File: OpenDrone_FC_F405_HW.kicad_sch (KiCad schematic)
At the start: 88 parts, among them J1 Conn_01x05, J11 Conn_01x05, J12 Conn_01x05, J13 Conn_01x02, J14 Conn_01x02, J16 Conn_01x05, J17 Conn_02x03_Odd_Even, J2 Conn_01x02, J3 Conn_01x02, J4 Conn_01x02, J5 Conn_01x02, J6 Conn_01x08, J7 Conn_01x02, J8 Conn_01x04, J9 Conn_01x02, U1 STM32F405RGTx, U2 TPS54331, U4 MPU6000, U5 HMC5883L, U6 BMP280, U7 TPS54331, U8 Board, Y2 8Mhz

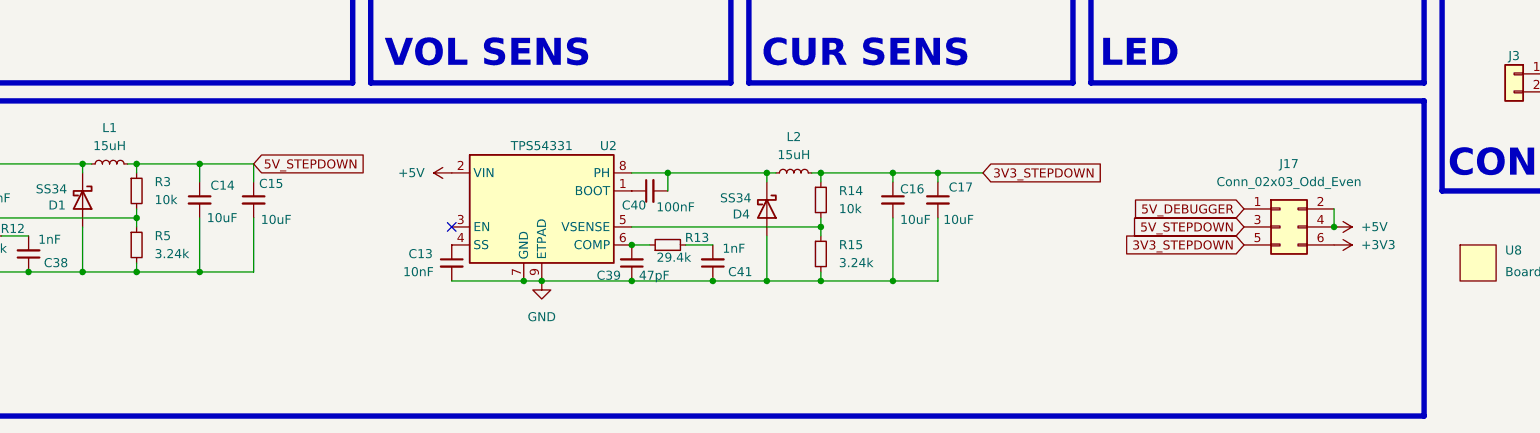
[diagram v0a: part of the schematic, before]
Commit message: update project
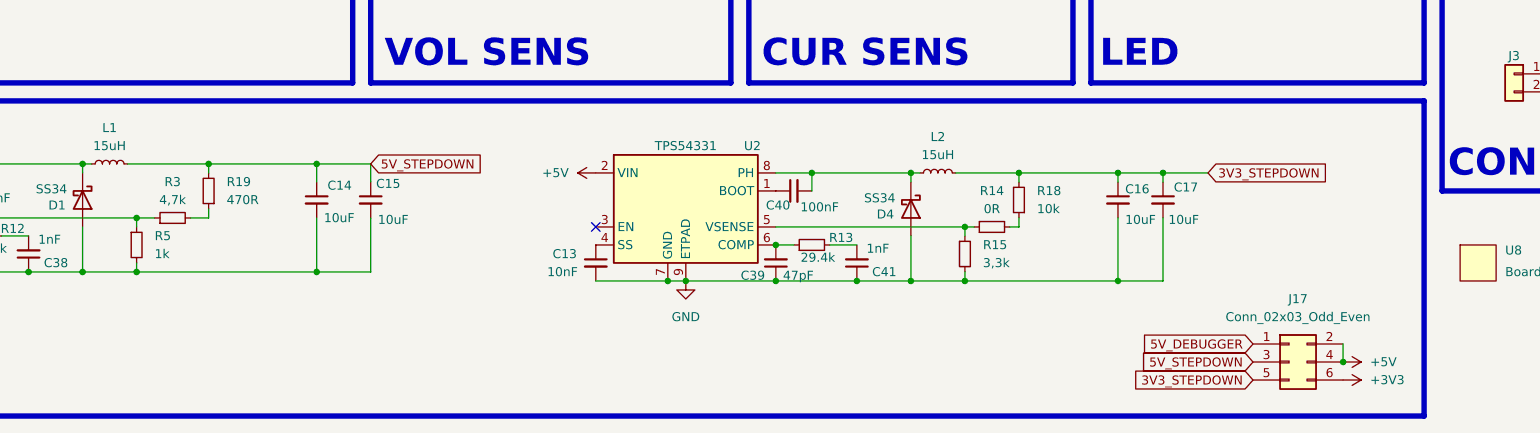
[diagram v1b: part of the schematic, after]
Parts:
- added R18: 10k, Resistor_SMD:R_0402_1005Metric, symbol Device:R_Small
- added R19: 470R, Resistor_SMD:R_0402_1005Metric, symbol Device:R_Small
- R14: value 10k -> 0R
- R15: value 3.24k -> 3,3k
- R3: value 10k -> 4,7k
- R5: value 3.24k -> 1k
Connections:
- net 3V3_STEPDOWN: now also R18.2; no longer R14.1
- net 5V_STEPDOWN: now also R19.2; no longer R3.1
- net at R15.1, U2.5 (VSENSE): now also R14.1; no longer R14.2
- net at R5.1, U7.5 (VSENSE): now also R3.1; no longer R3.2
- new net: R14.2, R18.1
- new net: R19.1, R3.2
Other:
- moved on the sheet: C13, C14, C15, C16, C17, C39, C40, C41, D4, J17, L2, R13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

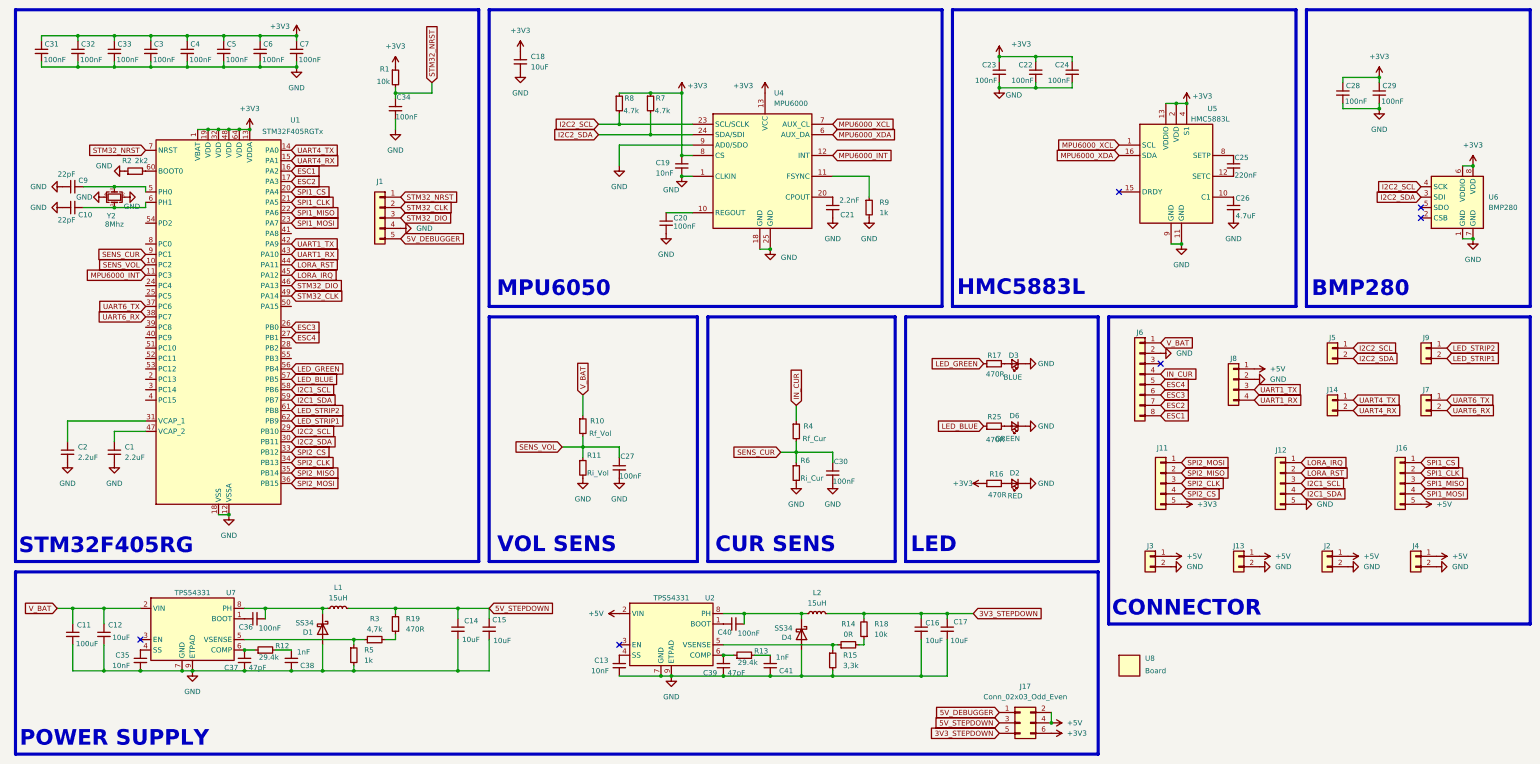
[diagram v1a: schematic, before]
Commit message: update project
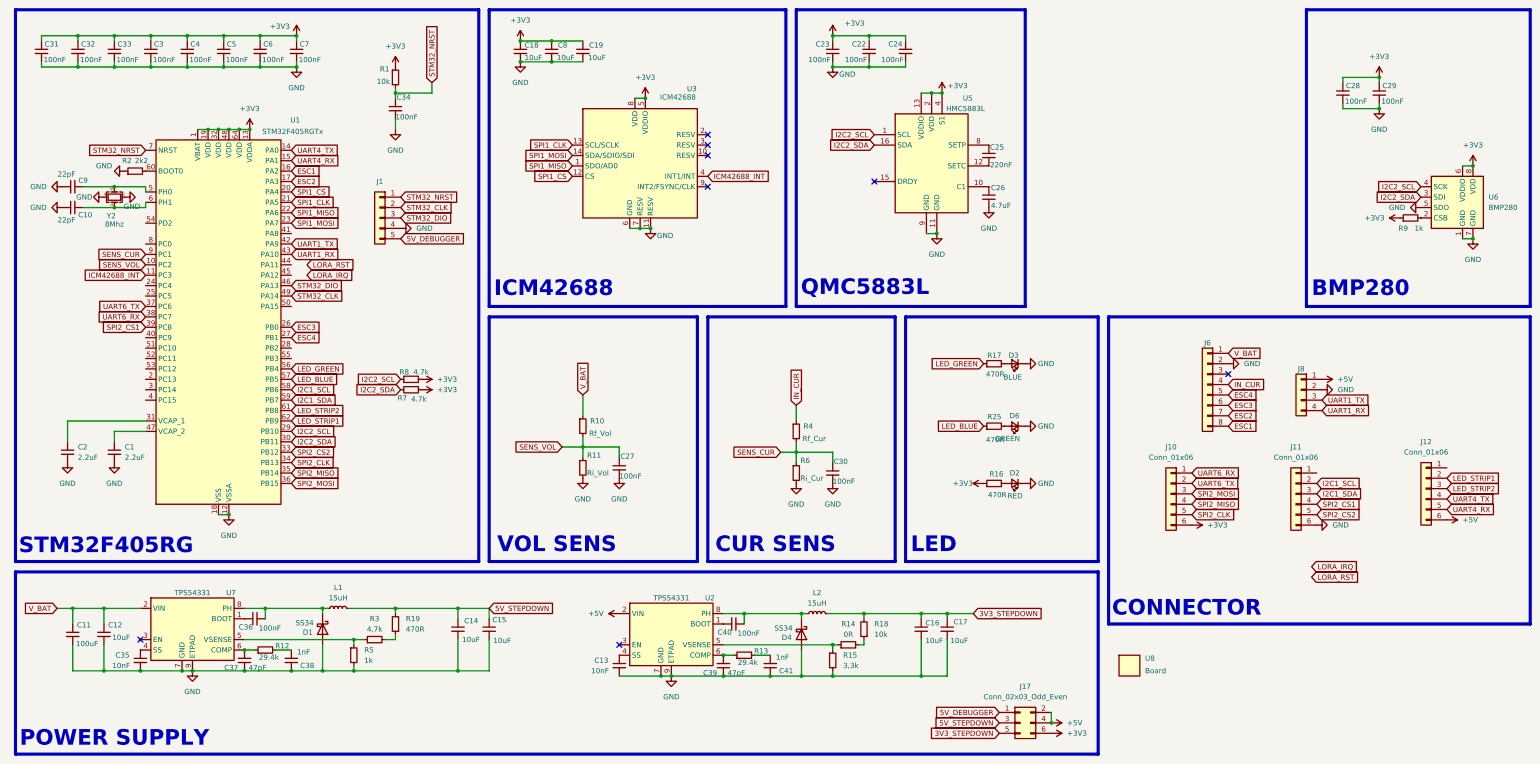
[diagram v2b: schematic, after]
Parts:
- removed C20: 100nF, Capacitor_SMD:C_0402_1005Metric, symbol Device:C_Small
- removed C21: 2.2nF, Capacitor_SMD:C_0402_1005Metric, symbol Device:C_Small
- removed J11, J12, J16: Conn_01x05, Footprint:Header_1x05_P2.00mm_Vertical, symbol Connector_Generic:Conn_01x05
- removed J13, J14, J2, J3, J4, J5, J7, J9: Conn_01x02, Footprint:HolePad_1x2, symbol Connector_Generic:Conn_01x02
- removed U4: MPU6000, Footprint:QFN-24-1EP_4x4mm_P0.5mm_EP2.15x2.15mm, symbol MPU6000:MPU6000
- added C8: 10uF, Capacitor_SMD:C_0402_1005Metric, symbol Device:C_Small
- added J10, J11, J12: Conn_01x06, Footprint:Header_1x06_P2.00mm_Vertical, symbol Connector_Generic:Conn_01x06
- added U3: ICM42688, Package_LGA:LGA-14_3x2.5mm_P0.5mm_LayoutBorder3x4y, symbol ICM42688:ICM42688
- C19: value 10nF -> 10uF
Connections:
- net MPU6000_XCL is gone; now on net I2C2_SCL: U5.1 (SCL)
- net MPU6000_XDA is gone; now on net I2C2_SDA: U5.16 (SDA)
- net +3V3: now also R8.2, R9.1, C8.1, J10.6 (Pin_6), U3.5 (VDDIO), U3.8 (VDD); no longer R8.1
- net +5V: now also J12.6 (Pin_6)
- net GND: now also U6.5 (SDO), C8.2, J11.6 (Pin_6), U3.11 (RESV), U3.6 (GND), U3.7 (RESV); no longer R9.2
- net I2C1_SCL: now also J11.2 (Pin_2)
- net I2C1_SDA: now also J11.3 (Pin_3)
- net I2C2_SCL: now also R8.1; no longer R8.2
- net LED_STRIP1: now also J12.2 (Pin_2)
- net LED_STRIP2: now also J12.3 (Pin_3)
- net LORA_IRQ: no longer U1.45 (PA12)
- net LORA_RST: no longer U1.44 (PA11)
- net SPI1_CLK: now also U3.13 (SCL/SCLK)
- net SPI1_CS: now also U3.12 (CS)
- net SPI1_MISO: now also U3.1 (SDO/AD0)
- net SPI1_MOSI: now also U3.14 (SDA/SDIO/SDI)
- net SPI2_CLK: now also J10.5 (Pin_5)
- net SPI2_MISO: now also J10.4 (Pin_4)
- net SPI2_MOSI: now also J10.3 (Pin_3)
- net UART4_RX: now also J12.5 (Pin_5)
- net UART4_TX: now also J12.4 (Pin_4)
- net UART6_RX: now also J10.1 (Pin_1)
- net UART6_TX: now also J10.2 (Pin_2)
- net at U6.2 (CSB): now also R9.2
- net SPI2_CS1: now reaches U1.39 (PC8)
- net SPI2_CS1: now also J11.4 (Pin_4)
- net MPU6000_INT renamed ICM42688_INT
- net ICM42688_INT: now also U3.4 (INT1/INT)
- net SPI2_CS renamed SPI2_CS2
- net SPI2_CS2: now also J11.5 (Pin_5)
- no-connect marks 6 -> 8
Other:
- note added: "ICM42688"
- note added: "QMC5883L"
- note removed: "HMC5883L"
- note removed: "MPU6050"
- moved on the sheet: C18, C22, C23, C24, C25, C26, J6, J8, R7, R8, R9, U5

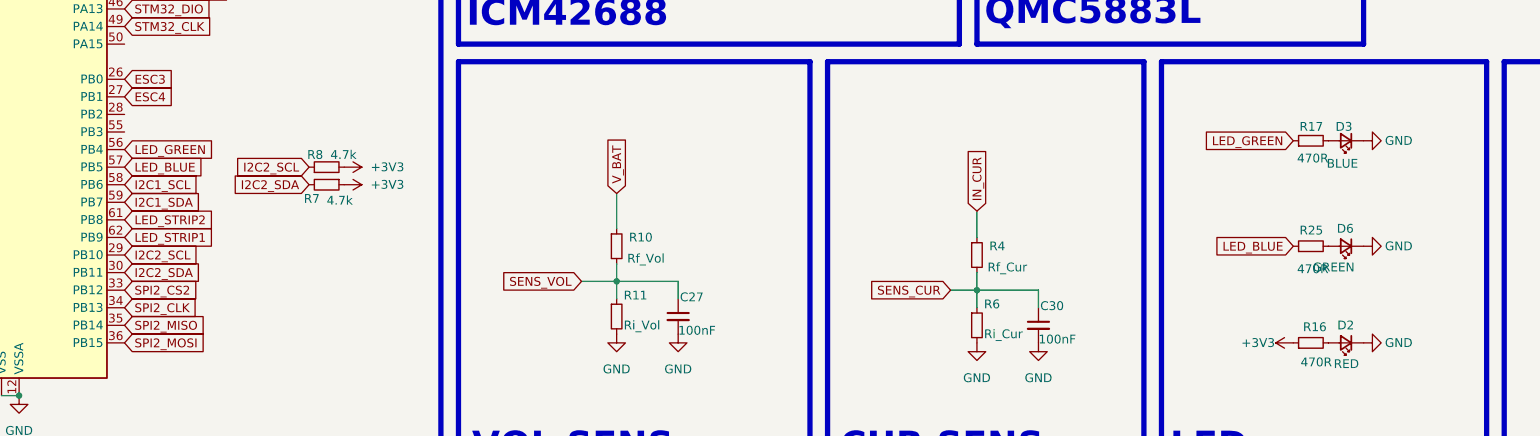
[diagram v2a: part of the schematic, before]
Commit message: update routing
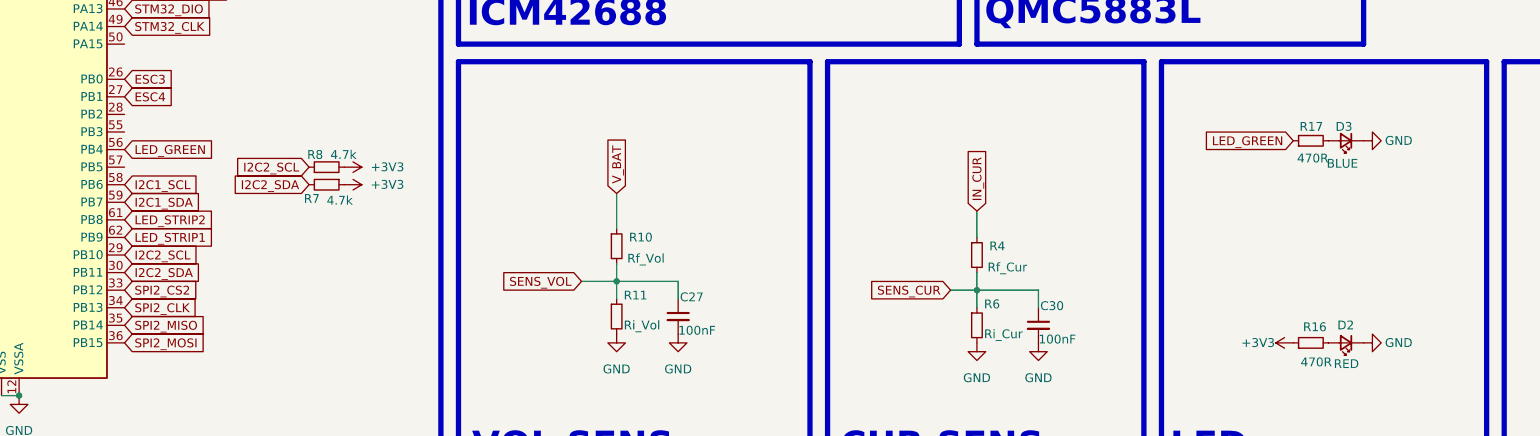
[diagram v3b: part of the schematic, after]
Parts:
- removed D6: GREEN, LED_SMD:LED_0402_1005Metric, symbol Device:LED_Small
- removed R25: 470R, Resistor_SMD:R_0402_1005Metric, symbol Device:R_Small
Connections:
- net LED_BLUE: no longer names the net of U1.57 (PB5)

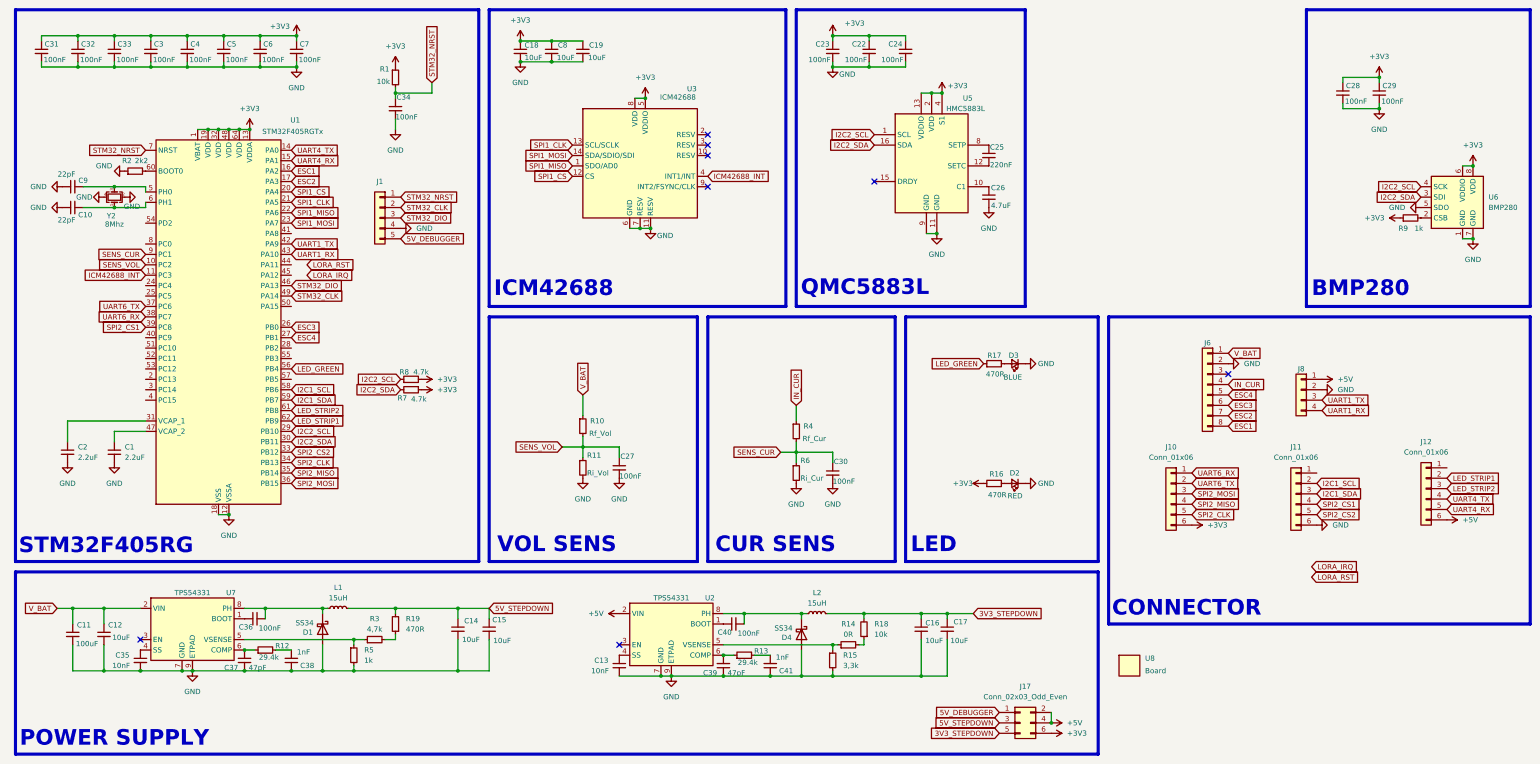
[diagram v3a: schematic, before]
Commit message: update routing
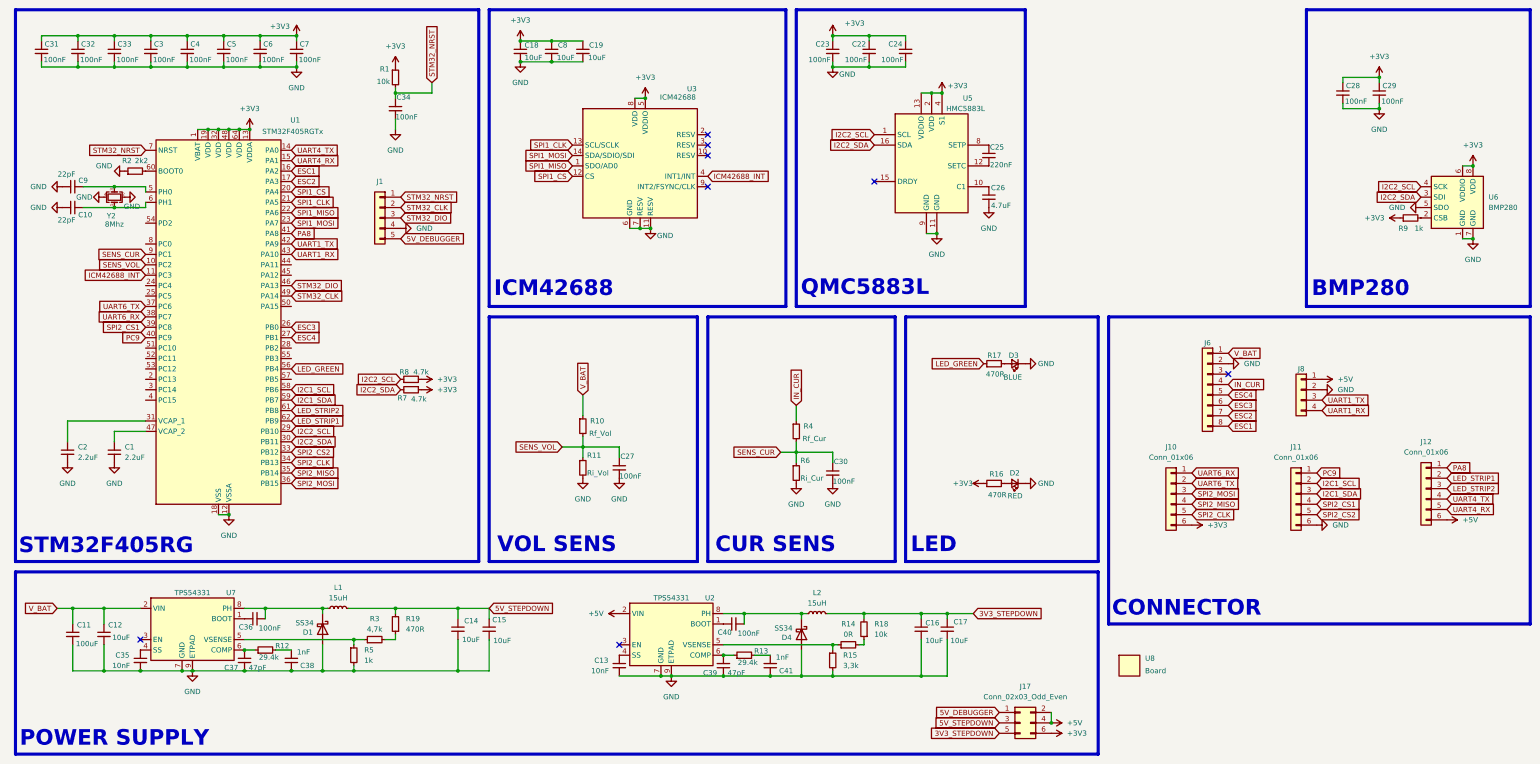
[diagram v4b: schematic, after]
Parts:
- U3: footprint Package_LGA:LGA-14_3x2.5mm_P0.5mm_LayoutBorder3x4y -> Footprint:LGA-14_3x2.5mm_P0.5mm
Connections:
- net PC9: now reaches U1.40 (PC9)
- net PC9: now also J11.1 (Pin_1)
- net PA8: now reaches U1.41 (PA8)
- net PA8: now also J12.1 (Pin_1)
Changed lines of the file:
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@@
 		)
 	)
-	(global_label "LORA_RST"
+	(global_label "PC9"
 		(shape input)
-		(at 330.2 152.4 0)
+		(at 331.47 127 0)
 		(fields_autoplaced yes)
 		(effects
@@
 		)
 		(property "Intersheetrefs" "${INTERSHEET_REFS}"
-			(at 342.3171 152.4 0)
+			(at 338.2047 127 0)
 			(effects
 				(font
@@
 		)
 	)
+	(global_label "PC9"
+		(shape input)
+		(at 45.72 93.98 180)
+		(fields_autoplaced yes)
+		(effects
+			(font
+				(size 1.27 1.27)
+			)
+			(justify right)
+		)
+		(property "Intersheetrefs" "${INTERSHEET_REFS}"
+			(at 38.9853 93.98 0)
+			(effects
+				(font
+					(size 1.27 1.27)
+				)
+				(justify right)
+				(hide yes)
+			)
+		)
+	)
 	(global_label "I2C1_SCL"
 		(shape input)
@@
 		)
 	)
-	(global_label "LORA_RST"
-		(shape input)
-		(at 85.09 76.2 0)
-		(fields_autoplaced yes)
-		(effects
-			(font
-				(size 1.27 1.27)
-			)
-			(justify left)
-		)
-		(property "Intersheetrefs" "${INTERSHEET_REFS}"
-			(at 97.2071 76.2 0)
-			(effects
-				(font
-					(size 1.27 1.27)
-				)
-				(justify left)
-				(hide yes)
-			)
-		)
-	)
 	(global_label "SPI2_CLK"
 		(shape input)
@@
 		)
 	)
-	(global_label "LORA_IRQ"
+	(global_label "PA8"
 		(shape input)
-		(at 330.2 149.86 0)
+		(at 363.22 125.73 0)
 		(fields_autoplaced yes)
 		(effects
@@
 		)
 		(property "Intersheetrefs" "${INTERSHEET_REFS}"
-			(at 342.0753 149.86 0)
+			(at 369.7733 125.73 0)
+			(effects
+				(font
+					(size 1.27 1.27)
+				)
+				(justify left)
+				(hide yes)
+			)
+		)
+	)
+	(global_label "PA8"
+		(shape input)
+		(at 81.28 68.58 0)
+		(fields_autoplaced yes)
+		(effects
+			(font
+				(size 1.27 1.27)
+			)
+			(justify left)
+		)
+		(property "Intersheetrefs" "${INTERSHEET_REFS}"
+			(at 87.8333 68.58 0)
 			(effects
 				(font
@@
 		)
 	)
-	(global_label "LORA_IRQ"
-		(shape input)
-		(at 85.09 78.74 0)
-		(fields_autoplaced yes)
-		(effects
-			(font
-				(size 1.27 1.27)
-			)
-			(justify left)
-		)
-		(property "Intersheetrefs" "${INTERSHEET_REFS}"
-			(at 96.9653 78.74 0)
-			(effects
-				(font
-					(size 1.27 1.27)
-				)
-				(justify left)
-				(hide yes)
-			)
-		)
-	)
 	(global_label "5V_STEPDOWN"
 		(shape input)
@@
 			)
 		)
-		(property "Footprint" "Package_LGA:LGA-14_3x2.5mm_P0.5mm_LayoutBorder3x4y"
+		(property "Footprint" "Footprint:LGA-14_3x2.5mm_P0.5mm"
 			(at 152.4 73.66 0)
 			(effects

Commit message: update setting
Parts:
- J6: footprint Footprint:Connector_XH_1x08_P1.25mm_Horizontal -> KiCad-Lib:Connector_XH_1x08_P1.25mm_Horizontal
- U3: footprint Footprint:LGA-14_3x2.5mm_P0.5mm -> KiCad-Lib:LGA-14_3x2.5mm_P0.5mm
- U5: footprint Footprint:QFN-16_3x3mm_P0.5mm -> KiCad-Lib:QFN-16_3x3mm_P0.5mm
- U6: footprint Footprint:LGA-8_2x2.5mm_P0.65mm -> KiCad-Lib:LGA-8_2x2.5mm_P0.65mm
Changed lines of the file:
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@@
 			)
 		)
-		(property "Footprint" "Footprint:LGA-8_2x2.5mm_P0.65mm"
+		(property "Footprint" "KiCad-Lib:LGA-8_2x2.5mm_P0.65mm"
 			(at 367.03 80.01 0)
 			(effects
@@
 			)
 		)
-		(property "Footprint" "Footprint:LGA-14_3x2.5mm_P0.5mm"
+		(property "Footprint" "KiCad-Lib:LGA-14_3x2.5mm_P0.5mm"
 			(at 152.4 73.66 0)
 			(effects
@@
 			)
 		)
-		(property "Footprint" "Footprint:QFN-16_3x3mm_P0.5mm"
+		(property "Footprint" "KiCad-Lib:QFN-16_3x3mm_P0.5mm"
 			(at 226.06 66.04 0)
 			(effects
@@
 			)
 		)
-		(property "Footprint" "Footprint:Connector_XH_1x08_P1.25mm_Horizontal"
+		(property "Footprint" "KiCad-Lib:Connector_XH_1x08_P1.25mm_Horizontal"
 			(at 304.8 105.41 0)
 			(effects
